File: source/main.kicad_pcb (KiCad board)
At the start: 2 copper layers, 0 parts

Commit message: Add basics
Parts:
- added D1: LED, lcsc:LED-SMD_L0.65-W0.35-P0.41_XL-0201SURC, F.Cu at (72.3, 40.0)
- added D2: LED, lcsc:LED-SMD_L0.65-W0.35-P0.41_XL-0201SURC, F.Cu at (72.3, 44.5)
- added P1: USB_Type_C_Receptacle_16_pin, lcsc:USB-C-SMD_TYPE-C-6PIN-2MD-073, F.Cu at (64.5, 41.3)
- added R1: 5.1kΩ, lcsc:R0402, F.Cu at (60.6, 47.9)
- added R2: 5.1kΩ, lcsc:R0402, F.Cu at (60.6, 50.1)
- added R3: 100Ω, lcsc:R0402, F.Cu at (60.6, 52.2)
- added R4: 100Ω, lcsc:R0402, F.Cu at (60.6, 54.4)

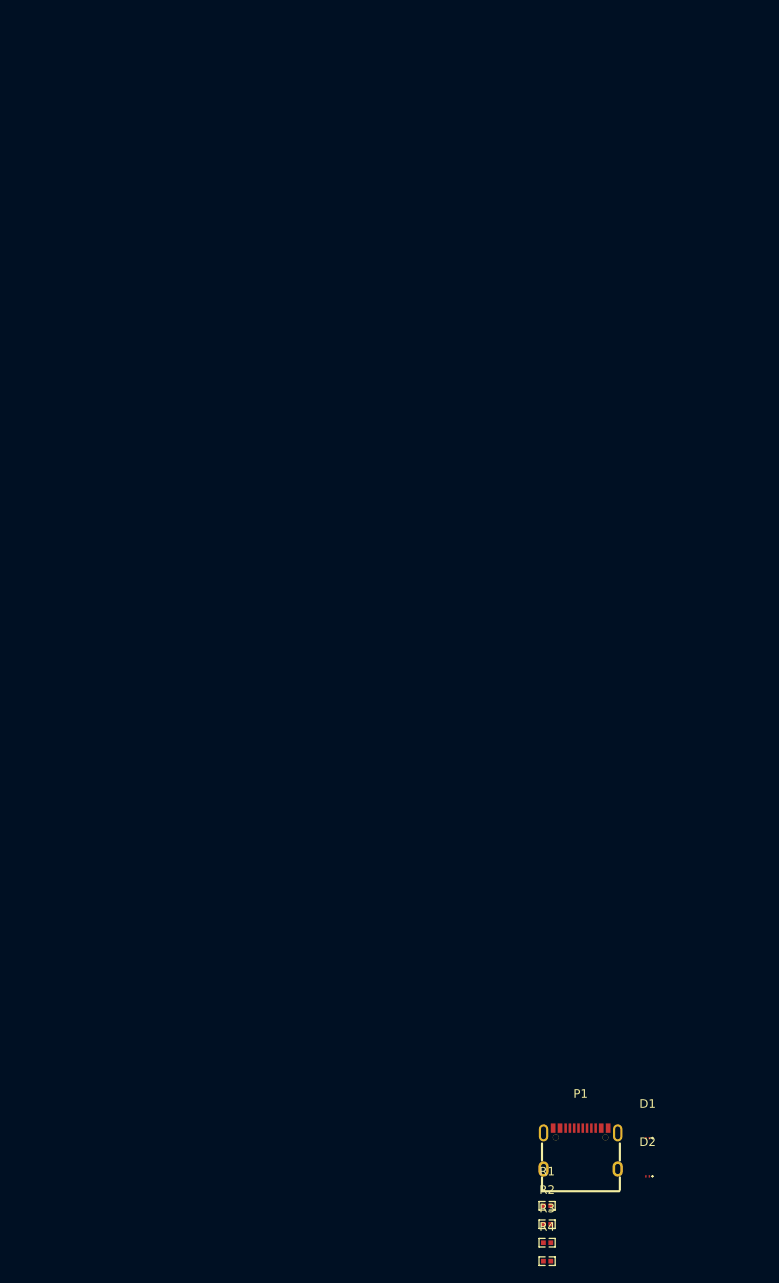
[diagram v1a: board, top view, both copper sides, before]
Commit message: Add WIP layout
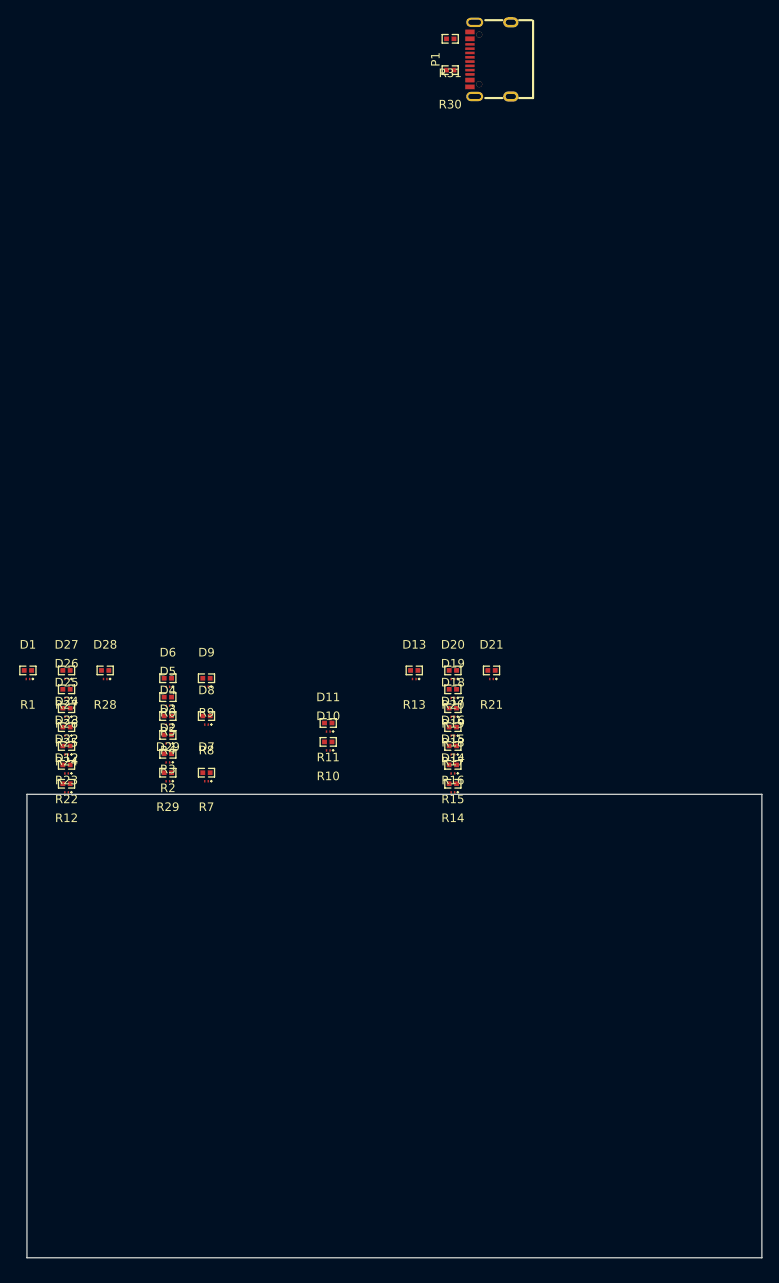
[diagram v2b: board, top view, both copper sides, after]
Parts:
- added D10: LED, lcsc:LED-SMD_L0.65-W0.35-P0.41_XL-0201SURC, F.Cu at (35.1, -5.11)
- added D11: LED, lcsc:LED-SMD_L0.65-W0.35-P0.41_XL-0201SURC, F.Cu at (35.1, -7.31)
- added D12: LED, lcsc:LED-SMD_L0.65-W0.35-P0.41_XL-0201SURC, F.Cu at (4.61, -0.23)
- added D13: LED, lcsc:LED-SMD_L0.65-W0.35-P0.41_XL-0201SURC, F.Cu at (45.1, -13.4)
- added D14: LED, lcsc:LED-SMD_L0.65-W0.35-P0.41_XL-0201SURC, F.Cu at (49.6, -0.23)
- added D15: LED, lcsc:LED-SMD_L0.65-W0.35-P0.41_XL-0201SURC, F.Cu at (49.6, -2.43)
- added D16: LED, lcsc:LED-SMD_L0.65-W0.35-P0.41_XL-0201SURC, F.Cu at (49.6, -4.63)
- added D17: LED, lcsc:LED-SMD_L0.65-W0.35-P0.41_XL-0201SURC, F.Cu at (49.6, -6.83)
- added D18: LED, lcsc:LED-SMD_L0.65-W0.35-P0.41_XL-0201SURC, F.Cu at (49.6, -9.03)
- added D19: LED, lcsc:LED-SMD_L0.65-W0.35-P0.41_XL-0201SURC, F.Cu at (49.6, -11.2)
- added D20: LED, lcsc:LED-SMD_L0.65-W0.35-P0.41_XL-0201SURC, F.Cu at (49.6, -13.4)
- added D21: LED, lcsc:LED-SMD_L0.65-W0.35-P0.41_XL-0201SURC, F.Cu at (54.1, -13.4)
- added D22: LED, lcsc:LED-SMD_L0.65-W0.35-P0.41_XL-0201SURC, F.Cu at (4.61, -2.43)
- added D23: LED, lcsc:LED-SMD_L0.65-W0.35-P0.41_XL-0201SURC, F.Cu at (4.61, -4.63)
- added D24: LED, lcsc:LED-SMD_L0.65-W0.35-P0.41_XL-0201SURC, F.Cu at (4.61, -6.83)
- added D25: LED, lcsc:LED-SMD_L0.65-W0.35-P0.41_XL-0201SURC, F.Cu at (4.61, -9.03)
- added D26: LED, lcsc:LED-SMD_L0.65-W0.35-P0.41_XL-0201SURC, F.Cu at (4.61, -11.2)
- added D27: LED, lcsc:LED-SMD_L0.65-W0.35-P0.41_XL-0201SURC, F.Cu at (4.61, -13.4)
- added D28: LED, lcsc:LED-SMD_L0.65-W0.35-P0.41_XL-0201SURC, F.Cu at (9.11, -13.4)
- added D29: LED, lcsc:LED-SMD_L0.65-W0.35-P0.41_XL-0201SURC, F.Cu at (16.4, -1.52)
- added D3: LED, lcsc:LED-SMD_L0.65-W0.35-P0.41_XL-0201SURC, F.Cu at (16.4, -5.92)
- added D4: LED, lcsc:LED-SMD_L0.65-W0.35-P0.41_XL-0201SURC, F.Cu at (16.4, -8.12)
- added D5: LED, lcsc:LED-SMD_L0.65-W0.35-P0.41_XL-0201SURC, F.Cu at (16.4, -10.3)
- added D6: LED, lcsc:LED-SMD_L0.65-W0.35-P0.41_XL-0201SURC, F.Cu at (16.4, -12.5)
- added D7: LED, lcsc:LED-SMD_L0.65-W0.35-P0.41_XL-0201SURC, F.Cu at (20.9, -1.52)
- added D8: LED, lcsc:LED-SMD_L0.65-W0.35-P0.41_XL-0201SURC, F.Cu at (20.9, -8.12)
- added D9: LED, lcsc:LED-SMD_L0.65-W0.35-P0.41_XL-0201SURC, F.Cu at (20.9, -12.5)
- added R10: 100Ω, lcsc:R0402, F.Cu at (35.1, -6.11)
- added R11: 100Ω, lcsc:R0402, F.Cu at (35.1, -8.31)
- added R12: 100Ω, lcsc:R0402, F.Cu at (4.61, -1.23)
- added R13: 100Ω, lcsc:R0402, F.Cu at (45.1, -14.4)
- added R14: 100Ω, lcsc:R0402, F.Cu at (49.6, -1.23)
- added R15: 100Ω, lcsc:R0402, F.Cu at (49.6, -3.43)
- added R16: 100Ω, lcsc:R0402, F.Cu at (49.6, -5.63)
- added R17: 100Ω, lcsc:R0402, F.Cu at (49.6, -7.83)
- added R18: 100Ω, lcsc:R0402, F.Cu at (49.6, -10.0)
- added R19: 100Ω, lcsc:R0402, F.Cu at (49.6, -12.2)
- added R20: 100Ω, lcsc:R0402, F.Cu at (49.6, -14.4)
- added R21: 100Ω, lcsc:R0402, F.Cu at (54.1, -14.4)
- added R22: 100Ω, lcsc:R0402, F.Cu at (4.61, -3.43)
- added R23: 100Ω, lcsc:R0402, F.Cu at (4.61, -5.63)
- added R24: 100Ω, lcsc:R0402, F.Cu at (4.61, -7.83)
- added R25: 100Ω, lcsc:R0402, F.Cu at (4.61, -10.0)
- added R26: 100Ω, lcsc:R0402, F.Cu at (4.61, -12.2)
- added R27: 100Ω, lcsc:R0402, F.Cu at (4.61, -14.4)
- added R28: 100Ω, lcsc:R0402, F.Cu at (9.11, -14.4)
- added R29: 100Ω, lcsc:R0402, F.Cu at (16.4, -2.52)
- added R30: 5.1kΩ, lcsc:R0402, F.Cu at (49.3, -84.3)
- added R31: 5.1kΩ, lcsc:R0402, F.Cu at (49.3, -88.0)
- added R5: 100Ω, lcsc:R0402, F.Cu at (16.4, -11.3)
- added R6: 100Ω, lcsc:R0402, F.Cu at (16.4, -13.5)
- added R7: 100Ω, lcsc:R0402, F.Cu at (20.9, -2.52)
- added R8: 100Ω, lcsc:R0402, F.Cu at (20.9, -9.12)
- added R9: 100Ω, lcsc:R0402, F.Cu at (20.9, -13.5)
- R1, R2: value 5.1kΩ -> 100Ω
- moved P1 127.3 mm to (54.0, -85.6), turned to 90 degrees
- moved D1 89.8 mm to (0.11, -13.4)
- moved R1 86.9 mm to (0.11, -14.4), turned to 180 degrees
- moved R4 77.4 mm to (16.4, -9.12), turned to 180 degrees
- moved R3 73.8 mm to (16.4, -6.92), turned to 180 degrees
- moved D2 73.8 mm to (16.4, -3.72)
- moved R2 70.4 mm to (16.4, -4.72), turned to 180 degrees
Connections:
- D1 pad 1: D1-1-R3-1 -> D1-1-R1-1
- D1 pad 2: vbus -> D1-2-D10-2-D11-2-D12-2-D13-2-D14-2-D15-2-D16-2-D17-2-D18-2-D19-2-D2-2-D20-2-D21-2-D22-2-D23-2-D24-2-D25-2-D26-2-D27-2-D28-2-D29-2-D3-2-D4-2-D5-2-D6-2-D7-2-D8-2-D9-2
- D2 pad 1: D2-1-R4-1 -> D2-1-R2-1
- D2 pad 2: vbus -> D1-2-D10-2-D11-2-D12-2-D13-2-D14-2-D15-2-D16-2-D17-2-D18-2-D19-2-D2-2-D20-2-D21-2-D22-2-D23-2-D24-2-D25-2-D26-2-D27-2-D28-2-D29-2-D3-2-D4-2-D5-2-D6-2-D7-2-D8-2-D9-2
- P1 pad 11: vbus -> P1-11-P1-2
- P1 pad 2: vbus -> P1-11-P1-2
- P1 pad 4: P1-4-R1-1 -> P1-4-R30-1
- P1 pad 9: P1-9-R2-1 -> P1-9-R31-1
- R1 pad 1: P1-4-R1-1 -> D1-1-R1-1
- R1 pad 2: gnd -> R1-2-R10-2-R11-2-R12-2-R13-2-R14-2-R15-2-R16-2-R17-2-R18-2-R19-2-R2-2-R20-2-R21-2-R22-2-R23-2-R24-2-R25-2-R26-2-R27-2-R28-2-R29-2-R3-2-R4-2-R5-2-R6-2-R7-2-R8-2-R9-2
- R2 pad 1: P1-9-R2-1 -> D2-1-R2-1
- R2 pad 2: gnd -> R1-2-R10-2-R11-2-R12-2-R13-2-R14-2-R15-2-R16-2-R17-2-R18-2-R19-2-R2-2-R20-2-R21-2-R22-2-R23-2-R24-2-R25-2-R26-2-R27-2-R28-2-R29-2-R3-2-R4-2-R5-2-R6-2-R7-2-R8-2-R9-2
- R3 pad 1: D1-1-R3-1 -> D3-1-R3-1
- R3 pad 2: gnd -> R1-2-R10-2-R11-2-R12-2-R13-2-R14-2-R15-2-R16-2-R17-2-R18-2-R19-2-R2-2-R20-2-R21-2-R22-2-R23-2-R24-2-R25-2-R26-2-R27-2-R28-2-R29-2-R3-2-R4-2-R5-2-R6-2-R7-2-R8-2-R9-2
- R4 pad 1: D2-1-R4-1 -> D4-1-R4-1
- R4 pad 2: gnd -> R1-2-R10-2-R11-2-R12-2-R13-2-R14-2-R15-2-R16-2-R17-2-R18-2-R19-2-R2-2-R20-2-R21-2-R22-2-R23-2-R24-2-R25-2-R26-2-R27-2-R28-2-R29-2-R3-2-R4-2-R5-2-R6-2-R7-2-R8-2-R9-2
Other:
- board outline added: 85.6 x 54 mm
